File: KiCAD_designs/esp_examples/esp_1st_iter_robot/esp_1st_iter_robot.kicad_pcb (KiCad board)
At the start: 2 copper layers, 22 parts, among them J1 B2B-PH-SM4-TBLFSN, J2 B2B-PH-SM4-TBLFSN, J3 Conn_01x02_Pin, J4 Conn_01x02_Pin, J5 Conn_01x03_Pin, Q1 AO3400A, SW1 KMR223G LFG, SW2 KMR223G LFG, U1 ESP-12F, U2 AMS1117-3.3, U3 CPT-9019S-SMT-TR

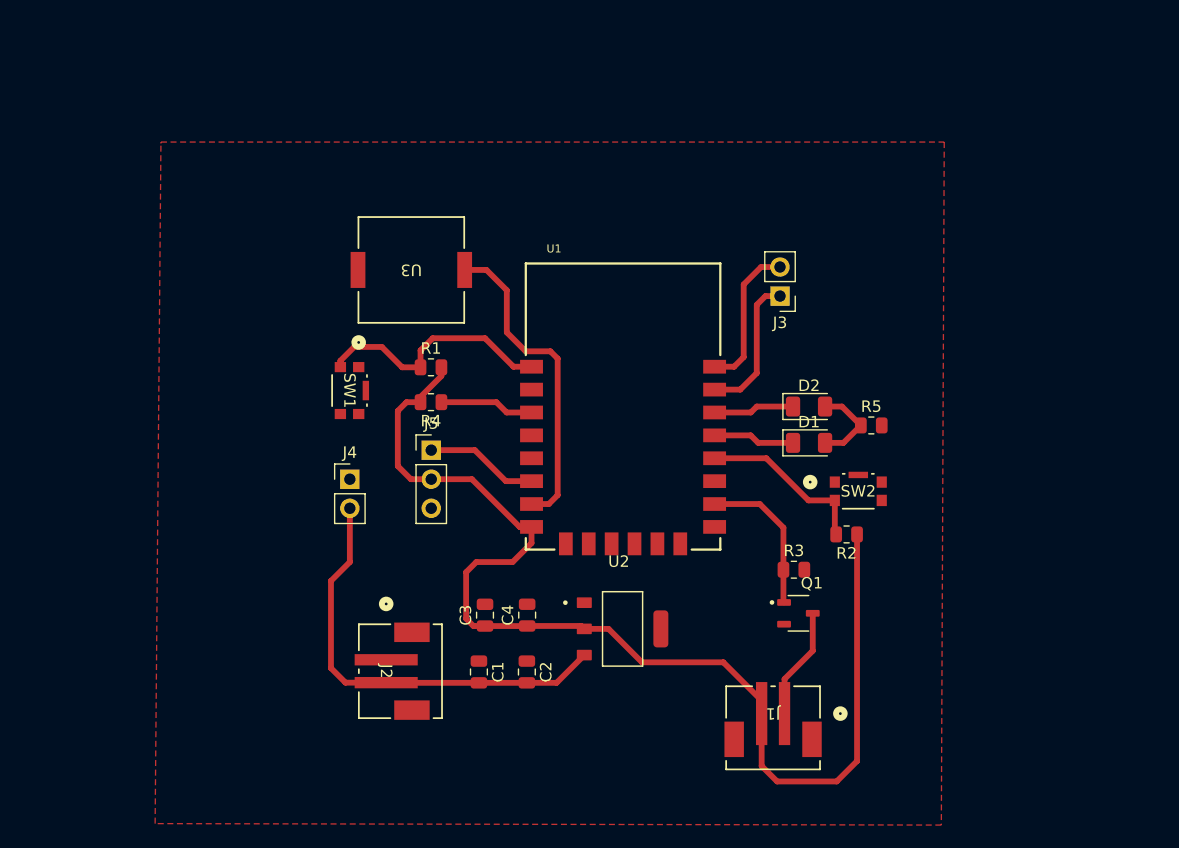
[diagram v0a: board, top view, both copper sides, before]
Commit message: esp_bot_fullRoute
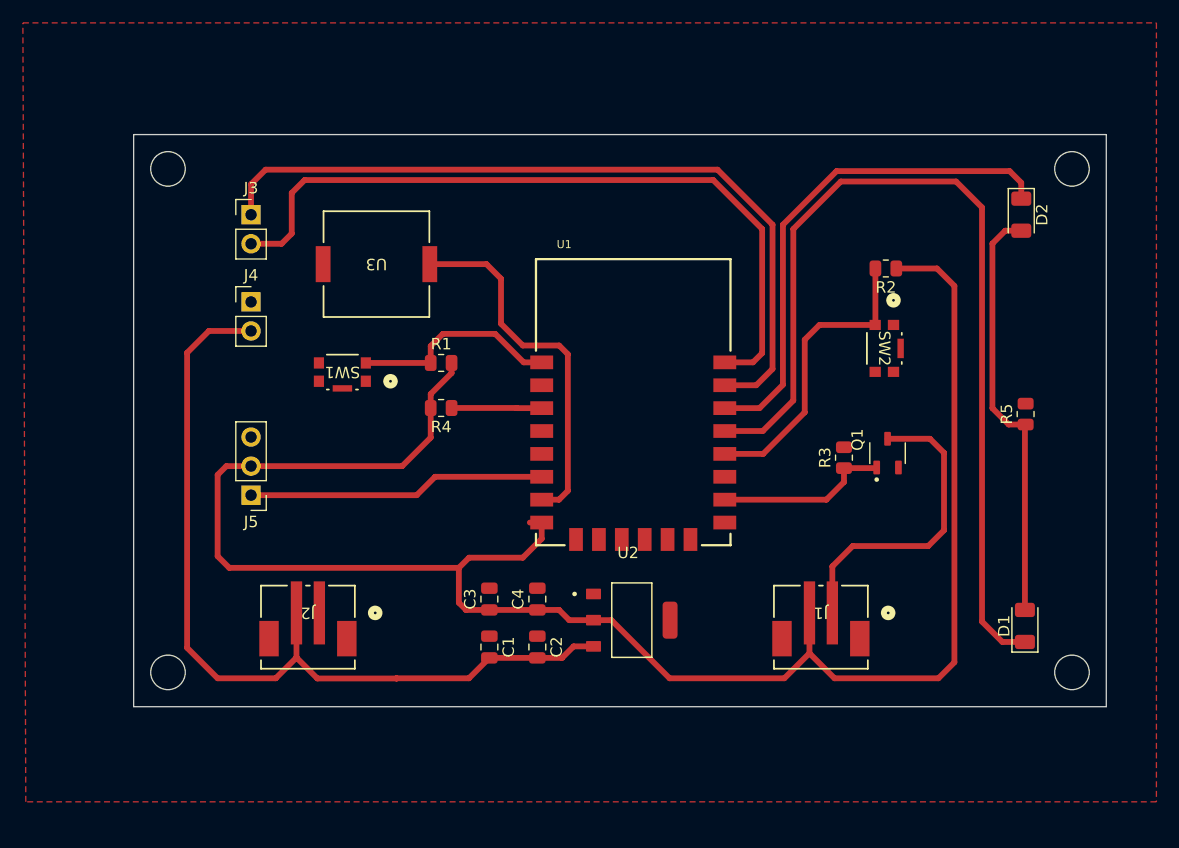
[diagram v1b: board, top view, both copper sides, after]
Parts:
- moved J3 46.8 mm to (40.3, 32.0), turned to 0 degrees
- moved D2 25.0 mm to (107.6, 32.0), turned to -90 degrees
- moved D1 24.7 mm to (107.9, 67.9), turned to 90 degrees
- moved R2 23.5 mm to (95.7, 36.7)
- moved J4 17.7 mm to (40.3, 39.6)
- moved J5 16.2 mm to (40.3, 56.5), turned to 180 degrees
- moved Q1 16.0 mm to (95.9, 52.8), turned to 90 degrees
- moved R5 13.5 mm to (108.0, 49.4), turned to 90 degrees
- moved SW2 12.7 mm to (95.6, 43.7), turned to -90 degrees
- moved R3 10.7 mm to (92.1, 53.2), turned to 90 degrees
- moved J1 9.74 mm to (90.1, 68.0)
- moved J2 8.96 mm to (45.2, 68.0), turned to 180 degrees
- moved U3 3.09 mm to (51.2, 36.3)
- moved C2 2.36 mm to (65.3, 69.8)
- moved C1 2.36 mm to (61.1, 69.8)
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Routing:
- net Net-(D1-K): track 7.12 -> 81.9 mm
- net VCC: track 101.0 -> 160.2 mm
- net Net-(J3-Pin_1): track 12.6 -> 68.1 mm
- net Net-(J3-Pin_2): track 13.0 -> 65.3 mm
- net Net-(D2-K): track 7.07 -> 44.5 mm
- net Net-(J4-Pin_2): track 38.3 -> 75.4 mm
- net Net-(D1-A): track 7.57 -> 37.1 mm
- net Net-(J1-Pad1): track 9.79 -> 27.3 mm
- net /servo: track 9.89 -> 26.1 mm
- net Net-(U1-GPIO0): track 15.1 -> 26.5 mm
- net Net-(U1-GPIO13): track 28.0 -> 32.2 mm
- net Net-(U1-RST): track 21.4 -> 18.3 mm
- net /DC: track 13.4 -> 15.2 mm
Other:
- board outline added: 85 x 50 mm
